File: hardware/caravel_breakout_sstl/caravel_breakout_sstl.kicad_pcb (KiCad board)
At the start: 2 copper layers, 25.4 x 25.4 mm, 20 parts, among them J1 Conn_01x14_Female, J2 Conn_01x14_Female, J3 Conn_01x14_Female, J4 Conn_01x14_Female, T1 Logo, T2 Logo, U1 Caravel

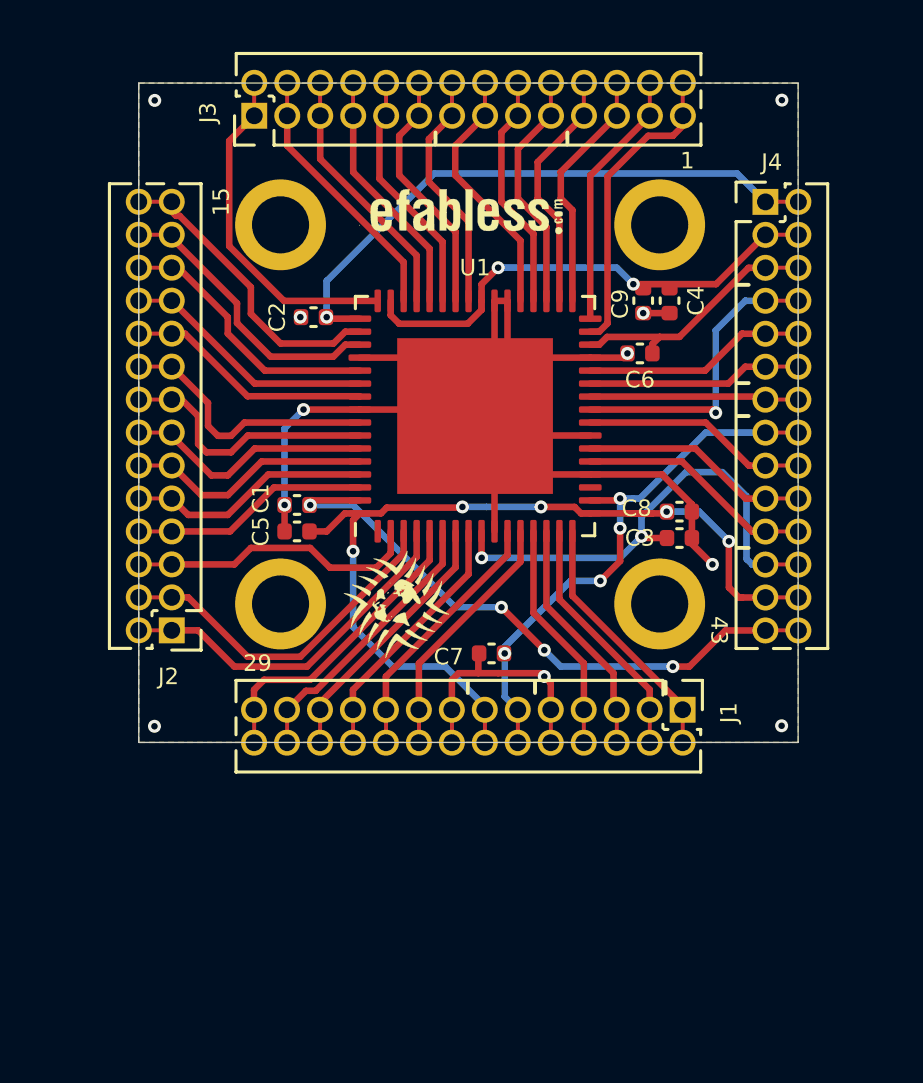
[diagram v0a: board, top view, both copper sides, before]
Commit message: Finish draft of Layout
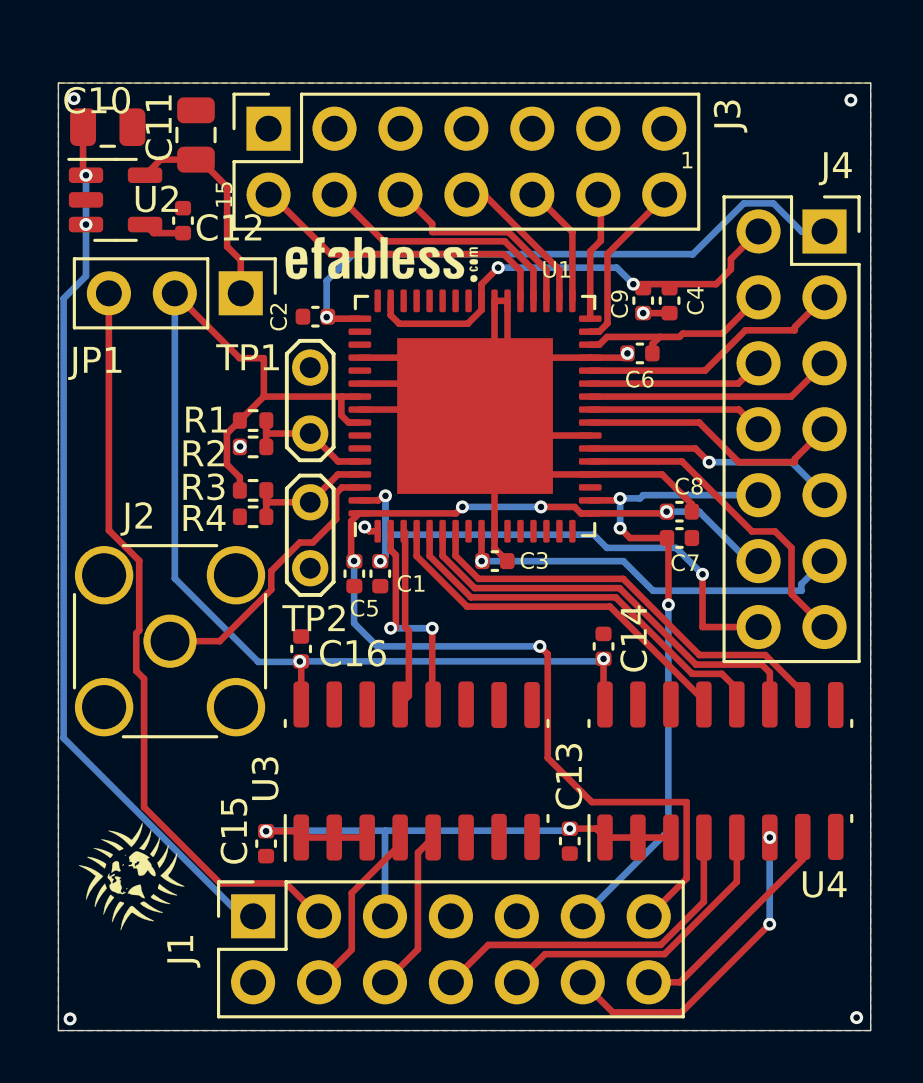
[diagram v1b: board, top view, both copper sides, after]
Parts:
- removed H1, H2, H3, H4: Positioning Holes, MountingHole:MountingHole_2.2mm_M2_ISO7380_Pad
- added C10: 10uf, Capacitor_SMD:C_0805_2012Metric, F.Cu at (119.2, 77.9)
- added C11: 10uf, Capacitor_SMD:C_0805_2012Metric, F.Cu at (122.6, 78.2)
- added C12: 0.1uf, Capacitor_SMD:C_0402_1005Metric, F.Cu at (122.1, 81.5)
- added C13: 0.1uf, Capacitor_SMD:C_0402_1005Metric, F.Cu at (137.0, 105.4)
- added C14: 0.1uf, Capacitor_SMD:C_0402_1005Metric, F.Cu at (138.3, 97.9)
- added C15: 0.1uf, Capacitor_SMD:C_0402_1005Metric, F.Cu at (125.3, 105.5)
- added C16: 0.1uf, Capacitor_SMD:C_0402_1005Metric, F.Cu at (126.7, 98.0)
- added JP1: Jumper_3_Open, Connector_PinHeader_2.54mm:PinHeader_1x03_P2.54mm_Vertical, F.Cu at (124.3, 84.3)
- added R1: 80.6ohm, Resistor_SMD:R_0402_1005Metric, F.Cu at (124.8, 89.2)
- added R2: 80.6ohm, Resistor_SMD:R_0402_1005Metric, F.Cu at (124.8, 90.2)
- added R3: 80.6ohm, Resistor_SMD:R_0402_1005Metric, F.Cu at (124.8, 91.9)
- added R4: 80.6ohm, Resistor_SMD:R_0402_1005Metric, F.Cu at (124.8, 92.9)
- added TP1: TestPoint_2Pole, TestPoint:TestPoint_2Pads_Pitch2.54mm_Drill0.8mm, F.Cu at (127.0, 89.7)
- added TP2: TestPoint_2Pole, TestPoint:TestPoint_2Pads_Pitch2.54mm_Drill0.8mm, F.Cu at (127.0, 92.3)
- added U2: LTC1844ES5-1.5, Package_TO_SOT_SMD:TSOT-23-5, F.Cu at (119.5, 80.7)
- added U3: SN74AVC4T245PW, custom_footprints:Texas_R-PDSO-G16, F.Cu at (131.1, 102.7)
- added U4: SN74AVC4T245PW, custom_footprints:Texas_R-PDSO-G16, F.Cu at (142.8, 102.7)
- J1, J3, J4: value Conn_01x14_Female -> Conn_02x07_Top_Bottom; footprint Connector_PinHeader_1.27mm:PinHeader_2x14_P1.27mm_Vertical -> Connector_PinSocket_2.54mm:PinSocket_2x07_P2.54mm_Vertical
- J2: value Conn_01x14_Female -> Conn_Coaxial; footprint Connector_PinHeader_1.27mm:PinHeader_2x14_P1.27mm_Vertical -> Connector_Coaxial:SMA_Amphenol_132134-16_Vertical
- moved J1 18.4 mm to (124.8, 108.3), turned to 90 degrees
- moved T1 14.6 mm to (120.1, 106.8)
- moved C7 8.49 mm to (141.2, 93.7), turned to 180 degrees
- moved C3 7.17 mm to (134.1, 94.6), turned to 0 degrees
- moved C1 4.16 mm to (129.7, 95.1), turned to 90 degrees
- moved T2 3.75 mm to (129.7, 83.0)
- moved C5 2.74 mm to (128.7, 95.1), turned to 90 degrees
- moved J4 2.54 mm to (146.8, 81.9)
- moved J3 0.74 mm to (125.4, 78.0)
- moved J2 0.42 mm to (121.6, 97.7), turned to 0 degrees
- moved C2 0.07 mm to (127.2, 85.2)
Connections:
- C3 pad 1: GND -> vdda2
- C3 pad 2: vdda2 -> GND
- J1 pad 1: mprj_io[37] -> vin_3v3
- J1 pad 10: GND -> prbs_clk_1_vin
- J1 pad 12: vccd -> prbs_clk_2_vin
- J1 pad 14: vddio -> ~{prsb_rst_vin}
- J1 pad 2: mprj_io[37] -> GND
- J1 pad 3: mprj_io[36] -> alt_vdd_1v5
- J1 pad 4: mprj_io[36] -> cfg_clk_vin
- J1 pad 5: mprj_io[35] -> cfg_vin
- J1 pad 6: mprj_io[35] -> cfg_din_vin
- J1 pad 7: mprj_io[34] -> GND
- J1 pad 8: mprj_io[34] -> prbs_clk_0_vin
- J2 pad 1: mprj_io[27] -> Net-(J2-Pad1)
- J2 pad 2: mprj_io[27] -> GND
- J3 pad 1: mprj_io[13] -> unconnected-(J3-Pad1)
- J3 pad 10: mprj_io[9] -> mprj_io[2]_SDI
- J3 pad 11: mprj_io[8] -> unconnected-(J3-Pad11)
- J3 pad 12: mprj_io[8] -> mprj_io[1]_SDO
- J3 pad 13: mprj_io[7] -> unconnected-(J3-Pad13)
- J3 pad 14: mprj_io[7] -> mprj_io[0]
- J3 pad 2: mprj_io[13] -> mprj_io[6]_ser_tx
- J3 pad 3: mprj_io[12] -> unconnected-(J3-Pad3)
- J3 pad 4: mprj_io[12] -> mprj_io[5]_ser_rx
- J3 pad 5: mprj_io[11] -> unconnected-(J3-Pad5)
- J3 pad 6: mprj_io[11] -> mprj_io[4]_SCK
- J3 pad 7: mprj_io[10] -> unconnected-(J3-Pad7)
- J3 pad 8: mprj_io[10] -> mprj_io[3]_CSB
- J3 pad 9: mprj_io[9] -> unconnected-(J3-Pad9)
- J4 pad 10: gpio -> vccd
- J4 pad 11: Caravel_D1 -> vdda2
- J4 pad 12: Caravel_D1 -> vddio
- J4 pad 13: Caravel_D0 -> ~{RST}
- J4 pad 14: Caravel_D0 -> vccd2
- J4 pad 2: vccd1 -> vdda1
- J4 pad 3: vdda1 -> gpio
- J4 pad 4: vdda1 -> vdda
- J4 pad 5: vdda -> Caravel_D0
- J4 pad 6: vdda -> Caravel_D1
- J4 pad 7: Caravel_SCK -> Caravel_CSB
- J4 pad 9: gpio -> xclk
- U1 pad 1: unconnected-(U1-Pad1) -> GND
- U1 pad 11: mprj_io[32] -> unconnected-(U1-Pad11)
- U1 pad 12: mprj_io[33] -> unconnected-(U1-Pad12)
- U1 pad 13: mprj_io[34] -> unconnected-(U1-Pad13)
- U1 pad 14: mprj_io[35] -> unconnected-(U1-Pad14)
- U1 pad 15: mprj_io[36] -> unconnected-(U1-Pad15)
- U1 pad 16: mprj_io[37] -> unconnected-(U1-Pad16)
- U1 pad 2: mprj_io[25] -> cfg_din
- U1 pad 3: mprj_io[26] -> cfg_clk
- U1 pad 4: mprj_io[27] -> prbs_clk_0
- U1 pad 41: mprj_io[7] -> unconnected-(U1-Pad41)
- U1 pad 42: mprj_io[8] -> unconnected-(U1-Pad42)
- U1 pad 43: mprj_io[9] -> unconnected-(U1-Pad43)
- U1 pad 44: mprj_io[10] -> unconnected-(U1-Pad44)
- U1 pad 45: mprj_io[11] -> unconnected-(U1-Pad45)
- U1 pad 46: mprj_io[12] -> unconnected-(U1-Pad46)
- U1 pad 48: mprj_io[13] -> unconnected-(U1-Pad48)
- U1 pad 5: mprj_io[28] -> prbs_clk_1
- U1 pad 50: mprj_io[14] -> unconnected-(U1-Pad50)
- U1 pad 51: mprj_io[15] -> unconnected-(U1-Pad51)
- U1 pad 53: mprj_io[16] -> unconnected-(U1-Pad53)
- U1 pad 54: mprj_io[17] -> GND
- U1 pad 55: mprj_io[18] -> analog_vdd
- U1 pad 57: mprj_io[19] -> analog_vdd
- U1 pad 58: mprj_io[20] -> GND
- U1 pad 59: mprj_io[21] -> unconnected-(U1-Pad59)
- U1 pad 6: mprj_io[29] -> prbs_clk_2
- U1 pad 60: mprj_io[22] -> tx_dq
- U1 pad 61: mprj_io[23] -> ~{tx_dq}
- U1 pad 62: mprj_io[24] -> Net-(J2-Pad1)
- U1 pad 7: mprj_io[30] -> ~{prbs_rst}
- U1 pad 8: mprj_io[31] -> unconnected-(U1-Pad8)
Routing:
- net analog_vdd: track 0.00 -> 47.9 mm, vias 0 -> 2
- net vin_3v3: track 0.00 -> 34.1 mm, vias 0 -> 2
- net alt_vdd_1v5: track 0.00 -> 28.9 mm
- net cfg_vin: track 0.00 -> 23.1 mm, vias 0 -> 2
- net ~{prbs_rst}: track 0.00 -> 17.0 mm
- net prbs_clk_2: track 0.00 -> 16.6 mm
- net prbs_clk_1: track 0.00 -> 15.5 mm
- net GND: track 68.7 -> 53.8 mm, vias 11 -> 8
- net prbs_clk_0: track 0.00 -> 14.5 mm
- net mprj_io[27]: track 13.8 -> 0.00 mm
- net prbs_clk_0_vin: track 0.00 -> 13.5 mm
- net mprj_io[26]: track 13.5 -> 0.00 mm
- net mprj_io[13]: track 13.1 -> 0.00 mm
- net prbs_clk_2_vin: track 0.00 -> 12.4 mm, vias 0 -> 2
- net mprj_io[28]: track 11.8 -> 0.00 mm
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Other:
- board size 25.4 x 25.4 mm -> 31.3 x 36.5 mm
- board text removed: "29"
- board text removed: "43"
